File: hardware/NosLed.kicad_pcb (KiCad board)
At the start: 2 copper layers, 25.4 x 61 mm, 23 parts, among them J101 LOAD, J102 PWM, J201 AC, U101 BP2876, U102 PC817

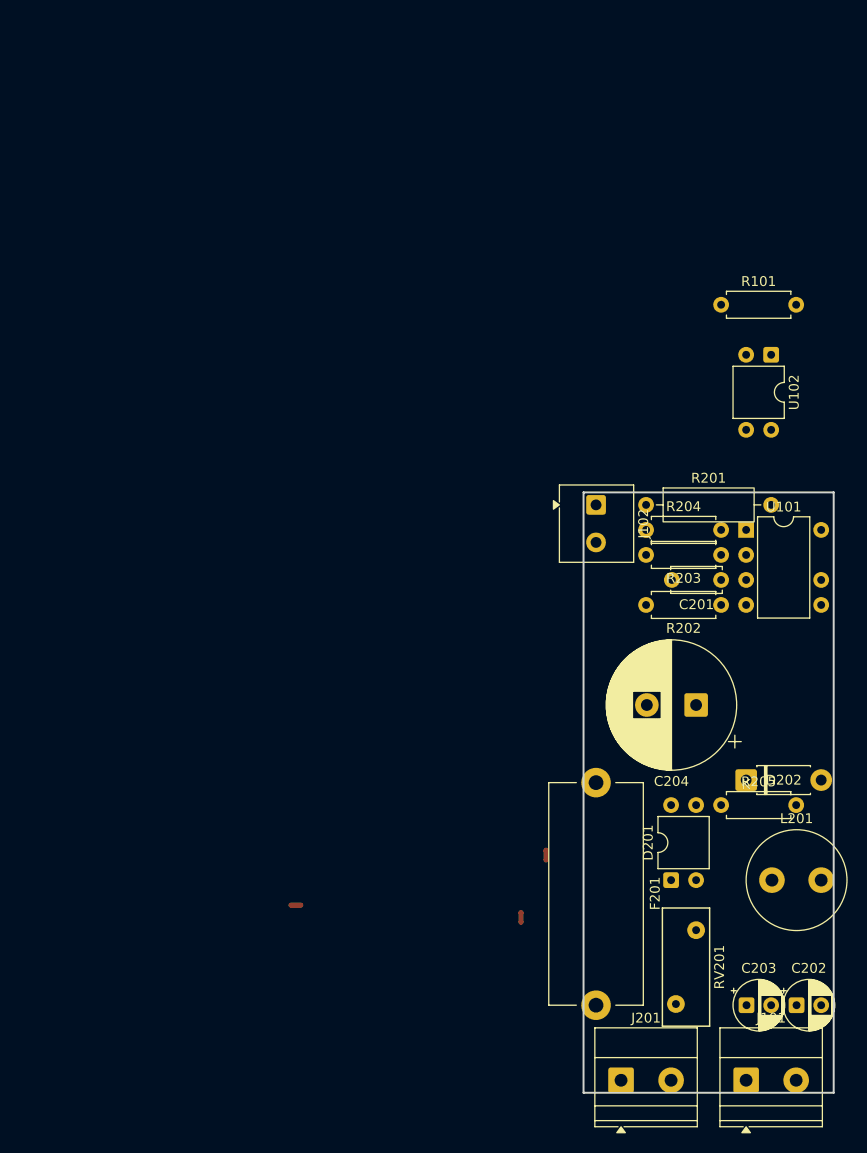
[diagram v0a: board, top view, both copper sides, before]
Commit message: AC Input
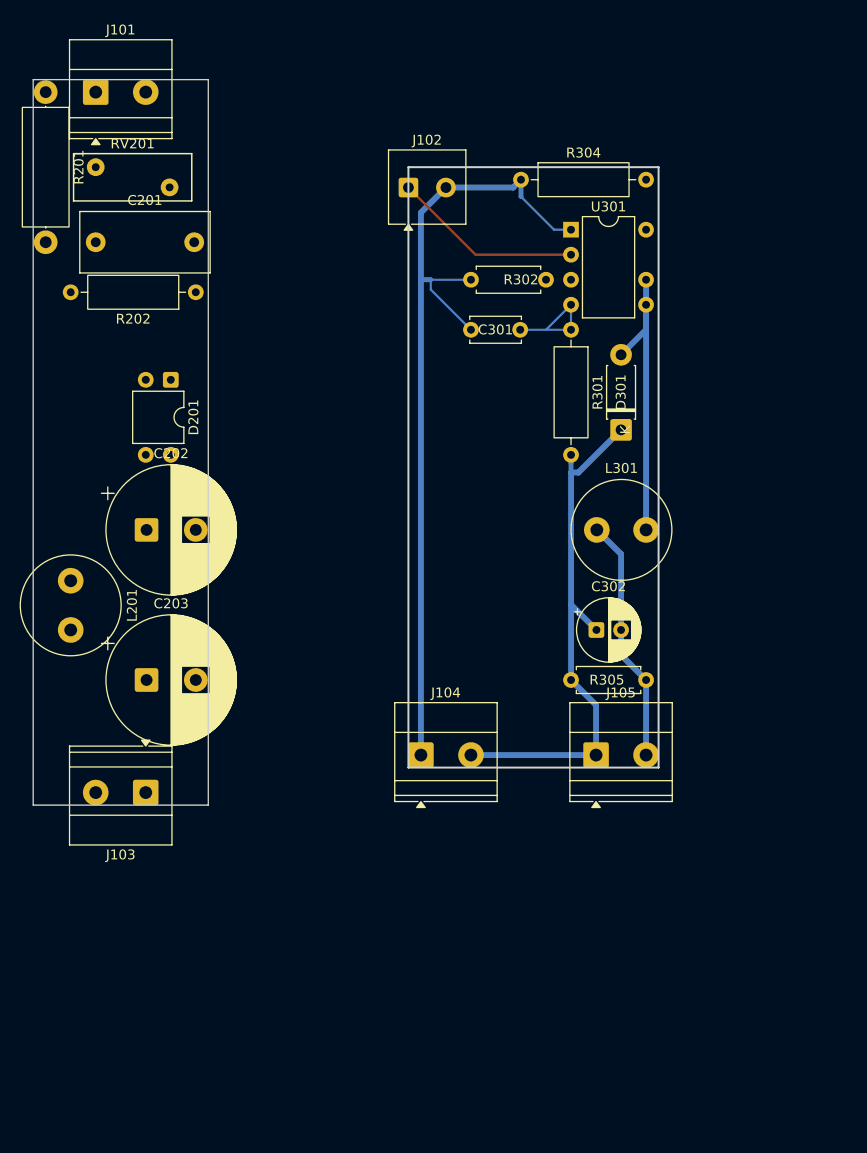
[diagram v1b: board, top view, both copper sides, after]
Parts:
- removed the C202 at (155.0, 149.9)
- removed F201: Fuse, Fuse:Fuseholder_Cylinder-5x20mm_Stelvio-Kontek_PTF78_Horizontal_Open
- removed J201: AC, TerminalBlock_Phoenix:TerminalBlock_Phoenix_MKDS-1,5-2-5.08_1x02_P5.08mm_Horizontal
- removed NT202: NetTie_2, NetTie:NetTie-2_SMD_Pad0.5mm
- removed R101: 330R, Resistor_THT:R_Axial_DIN0207_L6.3mm_D2.5mm_P7.62mm_Horizontal
- removed R204: 51K, Resistor_THT:R_Axial_DIN0207_L6.3mm_D2.5mm_P7.62mm_Horizontal
- removed U102: PC817, Package_DIP:DIP-4_W7.62mm
- added C201: MKP X2 275VAC, Capacitor_THT:C_Rect_L13.0mm_W6.0mm_P10.00mm_FKS3_FKP3_MKS4, F.Cu at (83.8, 72.4)
- added C203: 22uF 400v, Capacitor_THT:CP_Radial_D13.0mm_P5.00mm, F.Cu at (89.0, 116.8)
- added J101: AC, TerminalBlock_Phoenix:TerminalBlock_Phoenix_MKDS-1,5-2-5.08_1x02_P5.08mm_Horizontal, F.Cu at (83.8, 57.1)
- added J103: 380OUT, TerminalBlock_Phoenix:TerminalBlock_Phoenix_MKDS-1,5-2-5.08_1x02_P5.08mm_Horizontal, F.Cu at (88.9, 128.3)
- added J104: 380OUT, TerminalBlock_Phoenix:TerminalBlock_Phoenix_MKDS-1,5-2-5.08_1x02_P5.08mm_Horizontal, F.Cu at (116.8, 124.5)
- added L201: 1mH 0.5A, Inductor_THT:L_Radial_D10.0mm_P5.00mm_Fastron_07M, F.Cu at (81.3, 106.8)
- added NT303: NetTie_2, NetTie:NetTie-2_SMD_Pad0.5mm, B.Cu at (127.0, 67.3)
- added R201: Fusible 10R 1W, Resistor_THT:R_Axial_DIN0414_L11.9mm_D4.5mm_P15.24mm_Horizontal, F.Cu at (78.7, 57.1)
- added R202: 1M 0.5W, Resistor_THT:R_Axial_DIN0309_L9.0mm_D3.2mm_P12.70mm_Horizontal, F.Cu at (94.0, 77.5)
- C202: renamed from C204; value 33uF 400v -> 22uF 400v
- C302: renamed from C203; value 10uF 63v -> 10uF 100v; footprint Capacitor_THT:CP_Radial_D5.0mm_P2.50mm -> Capacitor_THT:CP_Radial_D6.3mm_P2.50mm
- D201: value MB10S -> MB10M
- NT301: renamed from NT201; moved to B.Cu
- NT302: renamed from NT203; moved to B.Cu
- R301: renamed from R202; footprint Resistor_THT:R_Axial_DIN0207_L6.3mm_D2.5mm_P7.62mm_Horizontal -> Resistor_THT:R_Axial_DIN0309_L9.0mm_D3.2mm_P12.70mm_Horizontal
- R302: renamed from R203; value 10K -> 27K
- moved RV201 97.6 mm to (91.3, 66.8), turned to 180 degrees
- moved D201 71.8 mm to (91.4, 86.4), turned to -90 degrees
- moved NT302 59.7 mm to (117.3, 76.2), turned to 180 degrees
- moved C202 58.6 mm to (89.0, 101.6), turned to 0 degrees
- moved NT301 45.9 mm to (132.1, 95.3)
- moved C302 41.0 mm to (134.7, 111.8)
- moved L301 39.8 mm to (134.7, 101.6)
- moved D301 37.8 mm to (137.2, 91.4), turned to 90 degrees
- moved J102 37.4 mm to (115.6, 66.8), turned to 0 degrees
- moved J105 36.4 mm to (134.6, 124.5)
- moved R304 35.4 mm to (127.0, 66.0)
- moved U301 35.3 mm to (132.1, 71.1)
- moved R302 33.1 mm to (129.5, 76.2)
- moved C301 32.6 mm to (126.9, 81.3)
- moved R301 31.8 mm to (132.1, 81.3), turned to -90 degrees
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- renumbered C201 to C301, D202 to D301, J101 to J105, L201 to L301, R201 to R304, R205 to R305, U101 to U301
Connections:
- net /BP2876/CS renamed /BP2876D/CS
- net /BP2876/DRAIN renamed /BP2876D/DRAIN
- C202 pad 1: /BP2876/LOAD+ -> Net-(D201-+)
- C202 pad 2: /BP2876/PWR_GND -> /BP2876D/PWR_GND
- C301 pad 2: Net-(U101-GND) -> Net-(C301-Pad2)
- C302 pad 1: /BP2876/LOAD+ -> /ACInput/380V
- C302 pad 2: Net-(C202-Pad1) -> /BP2876D/LOAD-
- D201 pad 1: /BP2876/AC_FUSE -> /ACInput/AC_N
- D201 pad 2: /BP2876/AC_L -> /ACInput/AC_L_FUSE
- D201 pad 3: /BP2876/LOAD+ -> Net-(D201-+)
- D201 pad 4: /BP2876/PWR_GND -> /BP2876D/PWR_GND
- D301 pad 1: /BP2876/LOAD+ -> /ACInput/380V
- J102 pad 1: /BP2876/HI_GND -> /BP2876D/PWM
- J102 pad 2: /BP2876/PWM -> /BP2876D/PWR_GND
- J105 pad 1: /BP2876/LOAD+ -> /ACInput/380V
- J105 pad 2: /BP2876/LOAD- -> /BP2876D/LOAD-
- L301 pad 1: /BP2876/LOAD- -> /BP2876D/LOAD-
- NT301 pad 2: /BP2876/LOAD+ -> /ACInput/380V
- NT302 pad 1: /BP2876/PWR_GND -> Net-(C301-Pad2)
- NT302 pad 2: Net-(U101-GND) -> /BP2876D/PWR_GND
- R302 pad 2: Net-(U101-GND) -> Net-(C301-Pad2)
- R304 pad 1: /BP2876/PWR_GND -> /BP2876D/PWR_GND
- R305 pad 1: /BP2876/LOAD+ -> /ACInput/380V
- R305 pad 2: /BP2876/LOAD- -> /BP2876D/LOAD-
- RV201 pad 1: /BP2876/AC_L -> /ACInput/AC_N
- RV201 pad 2: /BP2876/AC_FUSE -> /ACInput/AC_L_FUSE
- U301 pad 1: Net-(U101-GND) -> Net-(U301-GND)
- U301 pad 2: /BP2876/PWM -> /BP2876D/PWM
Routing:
- net /BP2876D/PWR_GND: track 0.00 -> 66.6 mm
- net /ACInput/380V: track 0.00 -> 53.0 mm
- net /BP2876D/DRAIN: track 0.00 -> 31.5 mm
- net /BP2876D/LOAD-: track 0.00 -> 24.9 mm
- net /BP2876D/PWM: track 0.00 -> 19.1 mm
- net Net-(U301-VCC): track 0.00 -> 11.3 mm
- net Net-(C301-Pad2): track 0.00 -> 10.8 mm
- net Net-(U301-GND): track 0.00 -> 6.47 mm
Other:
- board size 25.4 x 61 mm -> 63.5 x 73.7 mm
